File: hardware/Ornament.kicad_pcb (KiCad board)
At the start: 2 copper layers, 93.6 x 101.9 mm, 37 parts, among them J1 SWDIO, Q1 HL3400, Q2 HL3400, SW1 HX 0805-C2, U1 PY32F002BL15S7TU

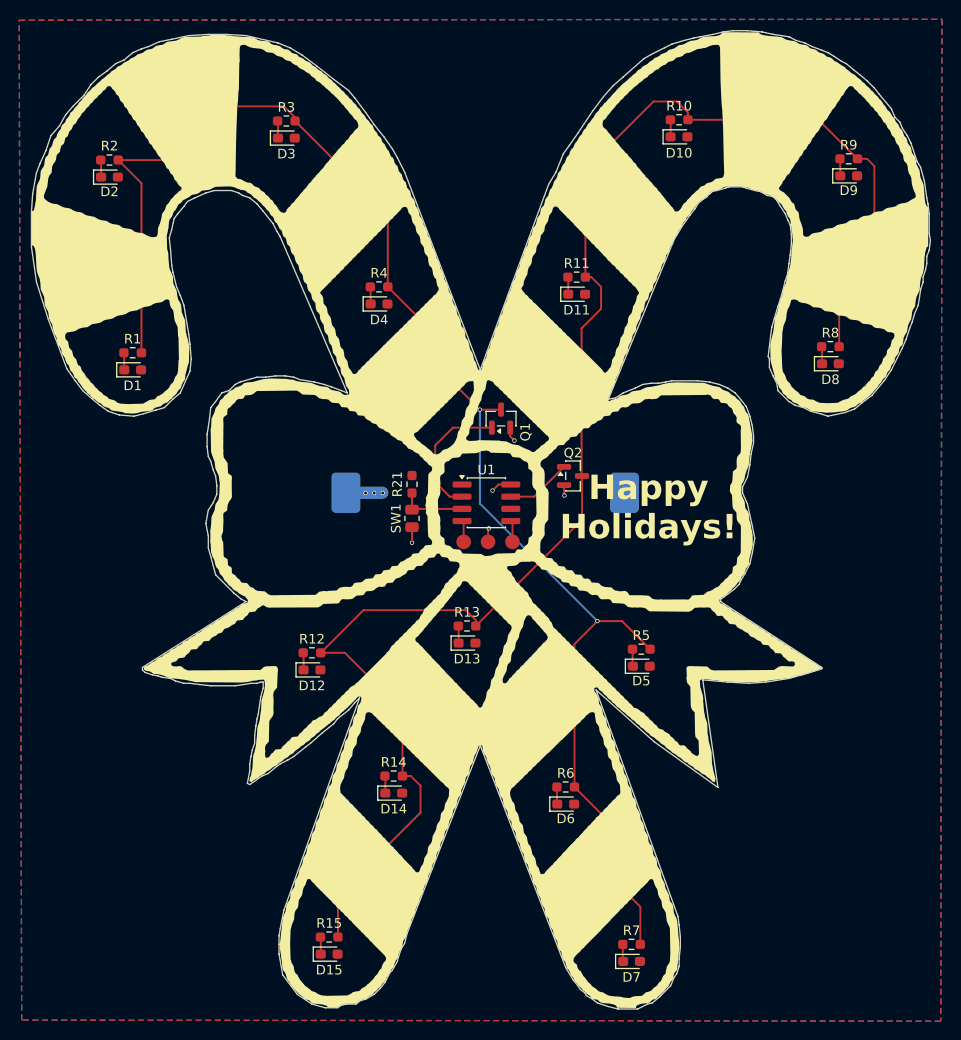
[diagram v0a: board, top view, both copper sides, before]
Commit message: init dev board
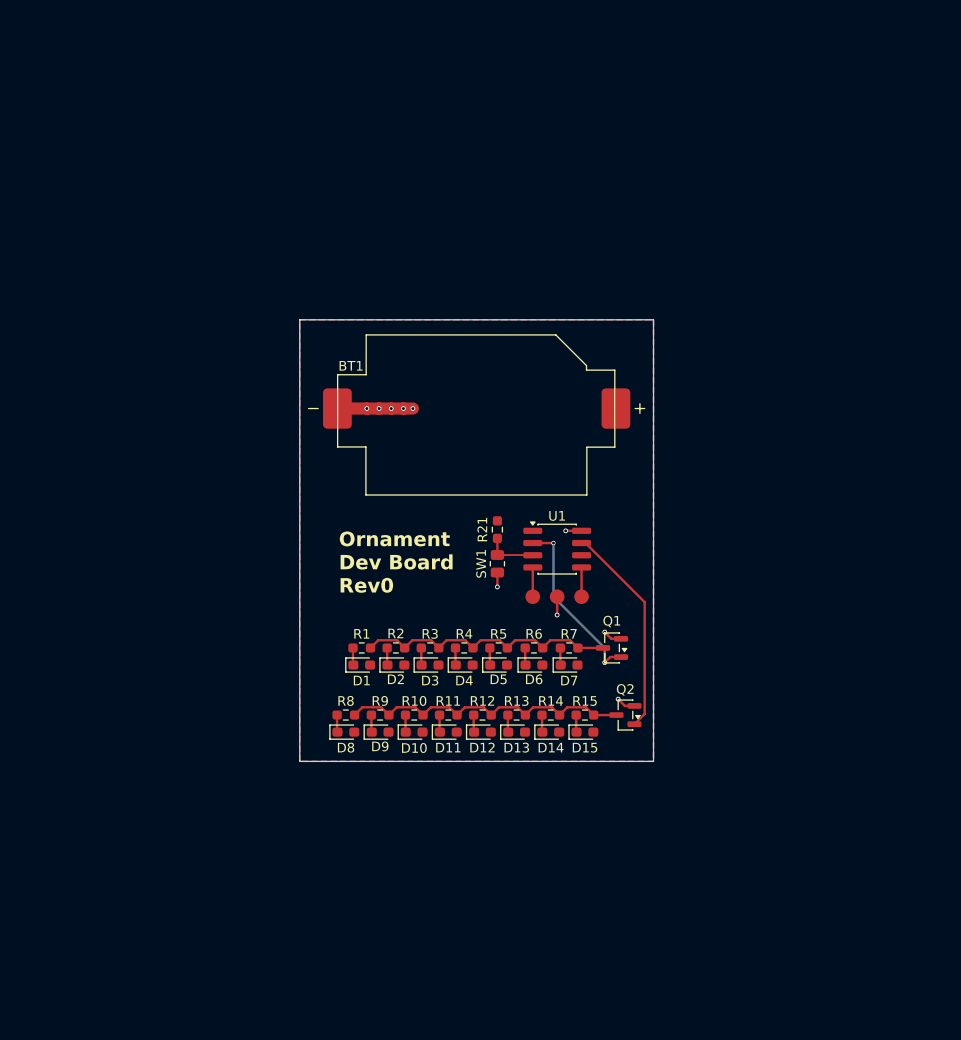
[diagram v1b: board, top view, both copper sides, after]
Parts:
- BT1: moved to F.Cu
- moved D9 75.7 mm to (138.0, 127.1)
- moved R9 75.7 mm to (138.0, 125.3)
- moved D10 67.8 mm to (141.6, 127.1)
- moved R10 67.8 mm to (141.6, 125.3)
- moved D8 63.4 mm to (134.4, 127.1)
- moved R8 63.4 mm to (134.4, 125.3)
- moved D2 58.9 mm to (139.7, 120.1)
- moved R2 58.9 mm to (139.7, 118.3)
- moved D3 56.9 mm to (143.2, 120.1)
- moved R3 56.9 mm to (143.2, 118.3)
- moved D11 47.5 mm to (145.1, 127.1)
- moved R11 47.5 mm to (145.1, 125.3)
- moved D1 38.9 mm to (136.1, 120.1)
- moved R1 38.9 mm to (136.1, 118.3)
- moved D4 38.6 mm to (146.8, 120.1)
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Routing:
- net Net-(Q2-D): track 169.0 -> 31.9 mm
- net Net-(Q1-D): track 154.1 -> 28.2 mm, vias 2 -> 0
- net /LED_B1: track 6.83 -> 22.3 mm
- net GND: track 8.21 -> 16.9 mm, vias 5 -> 10
- net /LED_B0: track 13.9 -> 18.7 mm, vias 0 -> 2
- net +3V: track 3.80 -> 0.00 mm, vias 3 -> 0
- net Net-(U1-PB0): track 6.97 -> 5.43 mm
- net (no net): vias 2 -> 0
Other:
- board size 93.6 x 101.9 mm -> 36.8 x 46 mm
- board text added: "Ornament Dev Board Rev0"
- board text removed: "From: Jacob, Sasha, Zhuzhu, & Wormy"
- board text removed: "Happy Holidays!"
- board text removed: "Ornament2026 Rev0"
